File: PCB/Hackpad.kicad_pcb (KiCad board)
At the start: 2 copper layers, 83.3 x 66.7 mm, 9 parts, among them SW1 SW_Push, SW2 SW_Push, SW3 SW_Push, SW4 SW_Push, U1 XIAO-RP2040-DIP

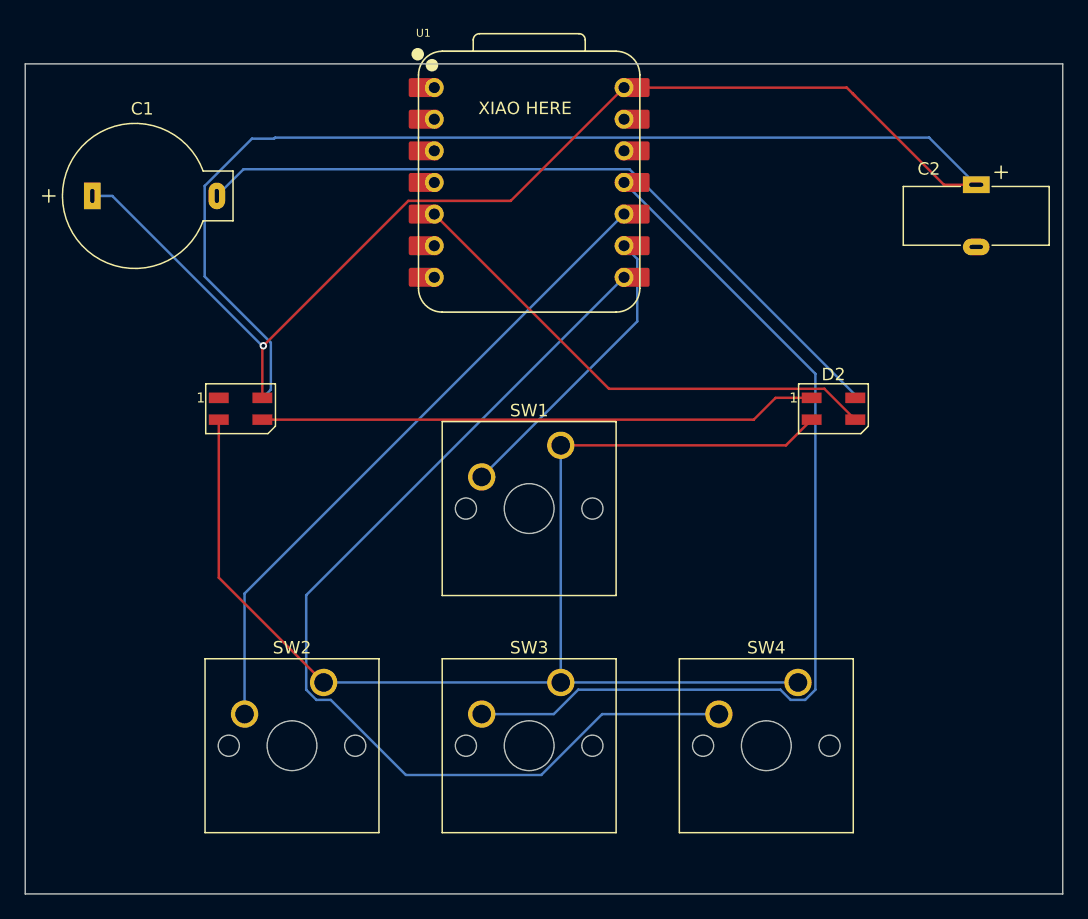
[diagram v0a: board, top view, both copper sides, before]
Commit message: fixed a lottta errors-ty meddy
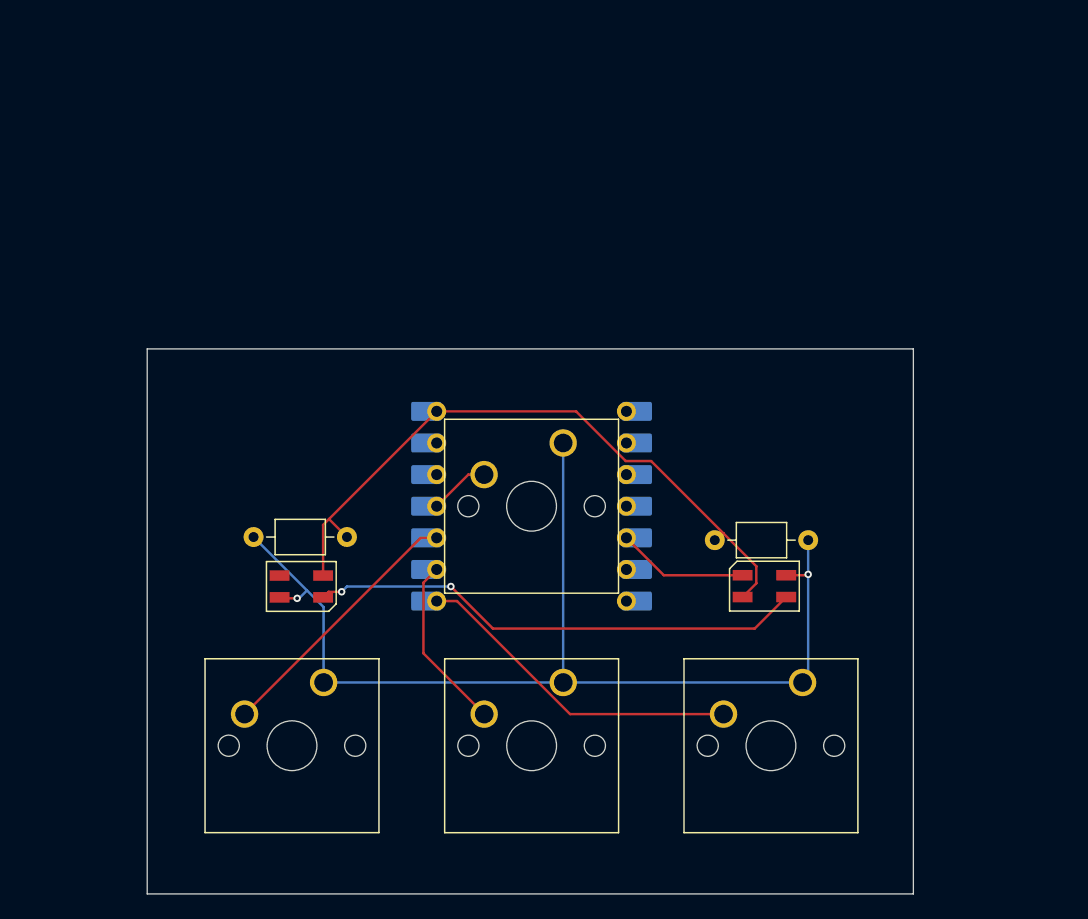
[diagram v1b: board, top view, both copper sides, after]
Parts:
- C1: footprint Capacitor_THT:DX_5R5HxxxxU_D11.5mm_P10.00mm -> Capacitor_THT:C_Axial_L3.8mm_D2.6mm_P7.50mm_Horizontal
- C2: footprint Capacitor_THT:DX_5R5VxxxxU_D11.5mm_P5.00mm -> Capacitor_THT:C_Axial_L3.8mm_D2.6mm_P7.50mm_Horizontal
- U1: moved to B.Cu
- moved C2 31.6 mm to (208.2, 83.5), turned to 180 degrees
- moved C1 30.3 mm to (163.6, 83.2)
- moved U1 26.0 mm to (185.9, 80.8), turned to 180 degrees
- moved SW3 19.2 mm to (188.5, 75.7)
- moved SW1 19.1 mm to (188.5, 94.9)
- moved D2 15.3 mm to (204.6, 87.2), turned to 180 degrees
- moved D1 15.1 mm to (167.4, 87.2)
- moved SW4 0.37 mm to (207.7, 94.9)
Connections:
- C1 pad 1: +5V -> GND
- C1 pad 2: Net-(D2-VDD) -> +5V
- C2 pad 1: Net-(D1-VDD) -> GND
- D1 pad 4: Net-(D1-VDD) -> +5V
- D2 pad 4: Net-(D2-VDD) -> +5V
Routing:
- net Net-(D1-VDD): track 84.7 -> 0.00 mm
- net Net-(U1-GPIO3/MOSI): track 75.4 -> 4.86 mm
- net Net-(D2-VDD): track 59.9 -> 0.00 mm
- net Net-(U1-GPIO1/RX): track 82.8 -> 26.8 mm
- net +5V: track 92.3 -> 53.7 mm, vias 1 -> 0
- net Net-(U1-GPIO4/MISO): track 52.8 -> 21.3 mm
- net Net-(D2-DIN): track 40.7 -> 10.6 mm
- net GND: track 102.8 -> 87.6 mm, vias 0 -> 2
- net Net-(U1-GPIO2/SCK): track 24.2 -> 14.1 mm
- net Net-(D1-DIN): track 44.8 -> 40.0 mm, vias 0 -> 2
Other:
- board size 83.3 x 66.7 mm -> 61.5 x 43.8 mm
- board text removed: "6-26-2025"
- board text removed: "Hackpad by Agniva/Knivier"
- board text removed: "XIAO HERE"
